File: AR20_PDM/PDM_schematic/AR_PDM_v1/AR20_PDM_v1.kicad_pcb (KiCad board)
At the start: 2 copper layers, 128 x 122 mm, 284 parts, among them J1 S_T_?, J2 1-776163-1, K1 DIPxx-1Cxx-51x, K2 DIPxx-1Cxx-51x, P1 B4B-PH-SM4-TB, Q1 BTS50025-1TAD, Q2 BTS50025-1TAD, Q3 BTS50025-1TAD, Q5 BTS50025-1TAD, Q6 BTS50025-1TAD, Q7 BTS50025-1TAD, Q8 BTS50025-1TAD, SW1 SW_DIP_x07, U1 ACM_2020, U10 N-MOS, U11 N-MOS, U12 P-MOS, U13 N-MOS, U14 N-MOS, U15 NMOS, U16 NMOS, U17 NMOS, U18 NMOS, U19 NMOS, U2 INA233, U20 NMOS, U21 NMOS, U22 NMOS, U23 NMOS, U24 NMOS, U25 NMOS, U26 NMOS, U27 NMOS, U28 NMOS, U29 INA233, U3 INA233, U30 INA233, U31 INA233, U32 Fet-P, U33 Fet-P, U34 Fet-P, U35 Fet-P, U36 Fet-P, U37 P-MOS-SIRA99DP-T1-GE3, U38 P-MOS-SIRA99DP-T1-GE3, U39 P-MOS-SIRA99DP-T1-GE3, U4 INA233, U40 P-MOS-SIRA99DP-T1-GE3, U41 P-MOS-SIRA99DP-T1-GE3, U5 INA233, U6 INA233, U7 INA233, U8 INA233, U9 TCA6424ARGJR

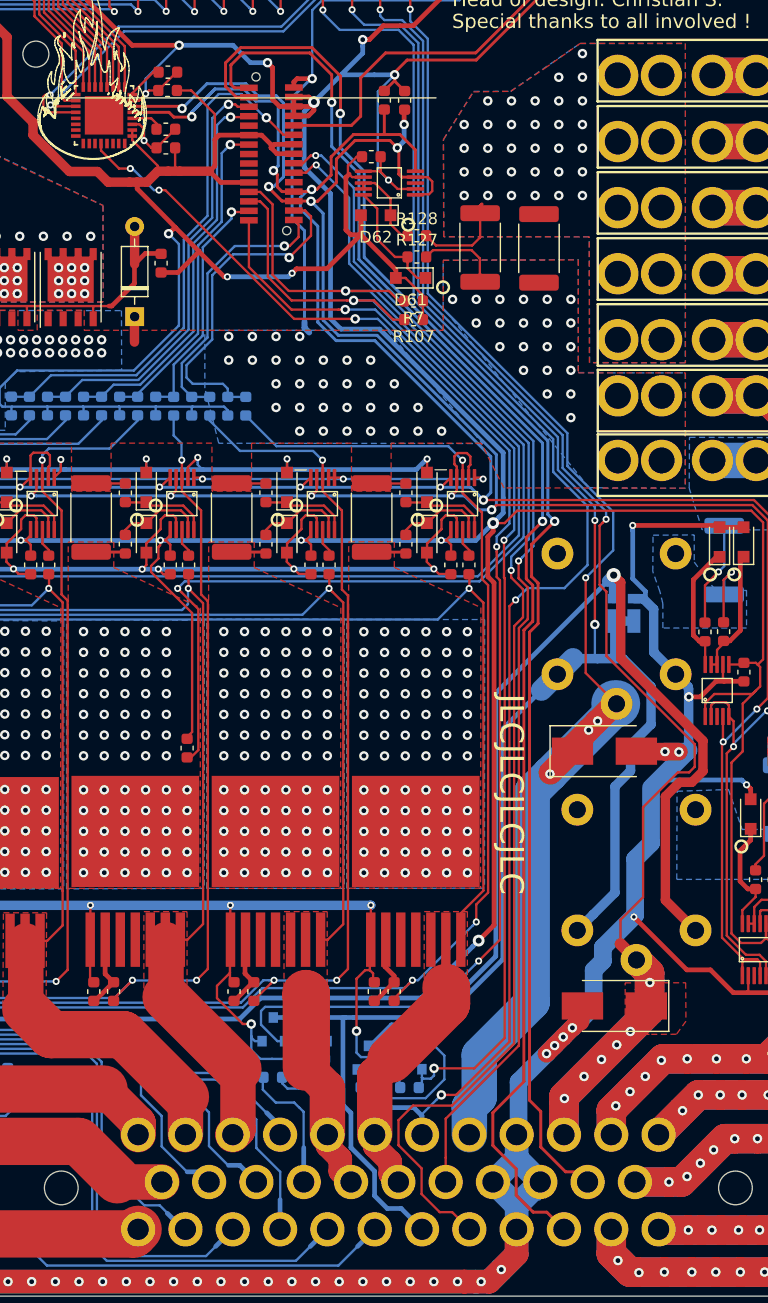
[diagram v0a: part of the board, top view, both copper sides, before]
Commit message: PDM V 3 Charlie Finished, awaiting final inspection
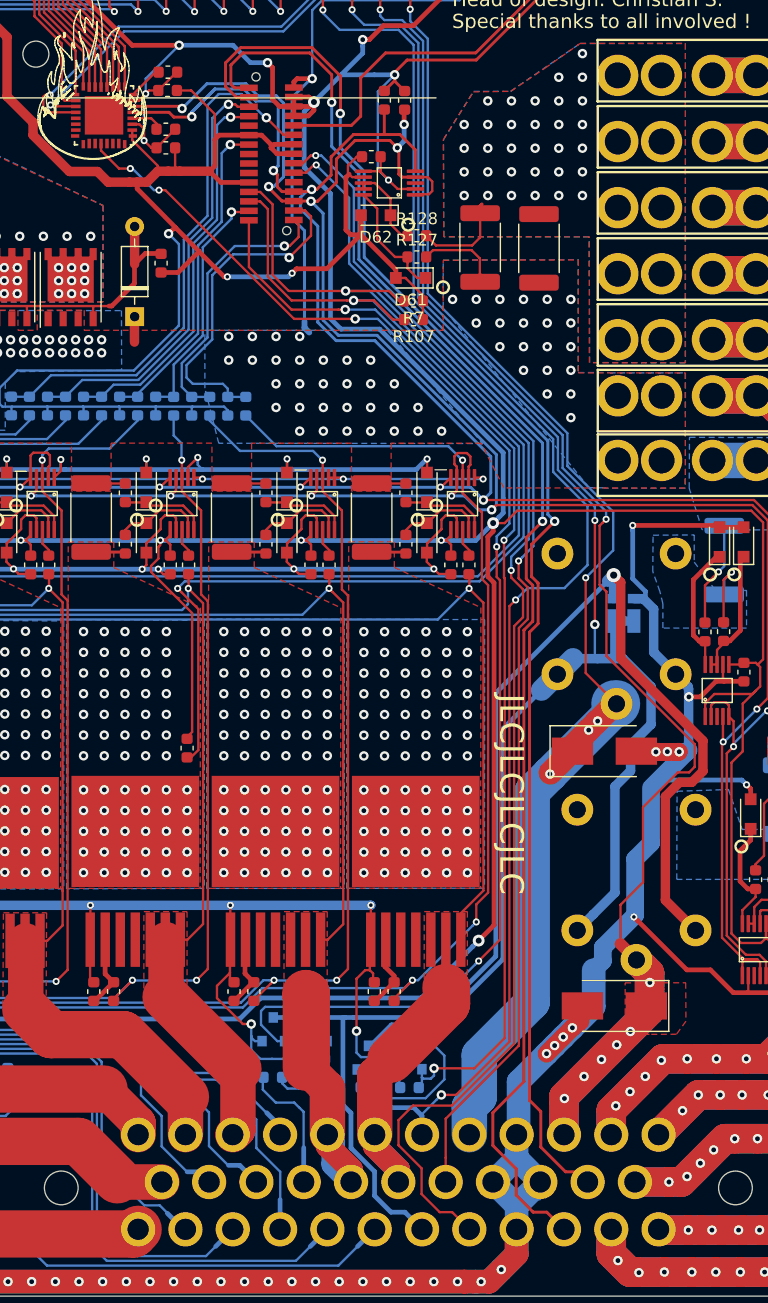
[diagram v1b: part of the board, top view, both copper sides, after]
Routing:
- net P6_OUT: track 223.5 -> 228.3 mm
- net P7_OUT: track 241.3 -> 245.1 mm
- net GND: track 1238.5 -> 1239.2 mm, vias 170 -> 171
